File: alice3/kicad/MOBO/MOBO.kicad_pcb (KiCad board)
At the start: 2 copper layers, 97.8 x 114.3 mm, 40 parts, among them CON1 SD_Card, P1 CONN_01X05, SW1 RESET, SW2 SOFT RESET, U1 LM2937-3.3, U2 VGA_daughter_board, U3 Propeller_P8X32A-D40, U4 24LC256, U5 Propeller_Plug, U6 MiniM4-D40, U7 DFROBOT_FTDI_BASIC, U8 Z80CPU, U9 KM681000BLP-7, Y1 5 MHz

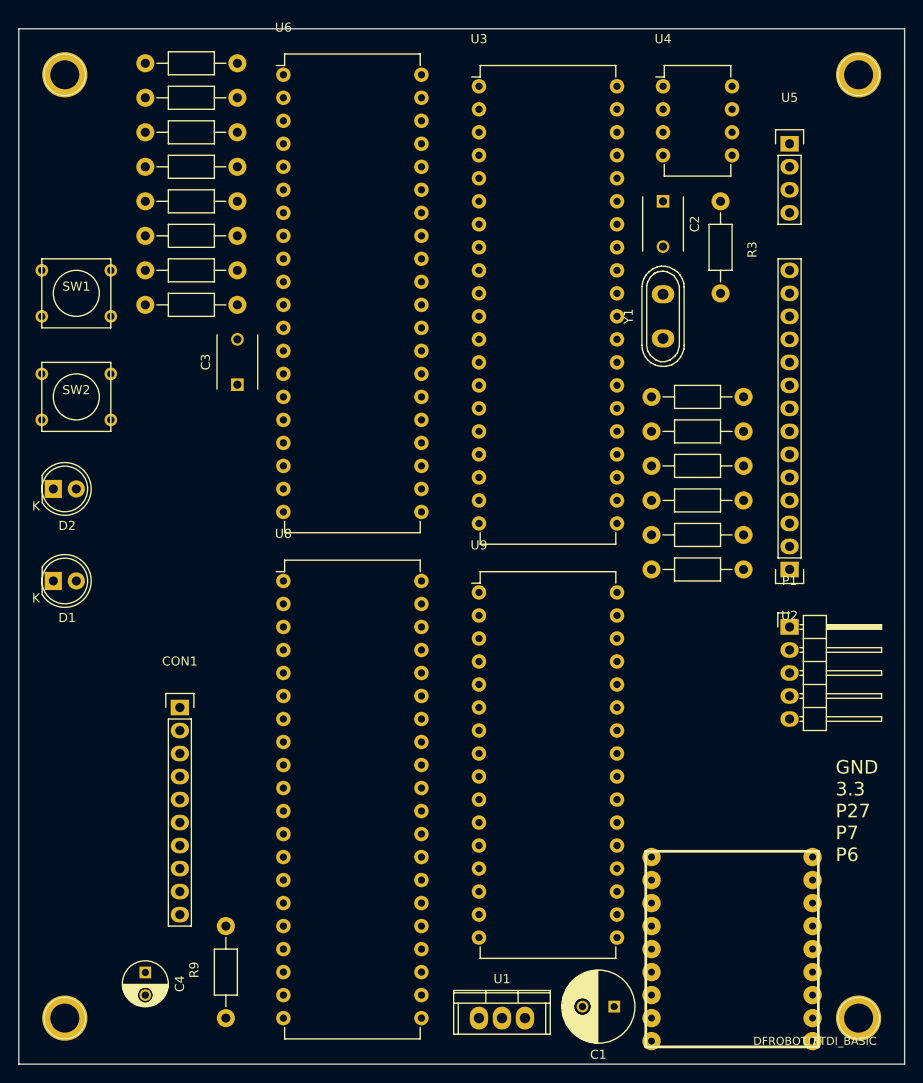
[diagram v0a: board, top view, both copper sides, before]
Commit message: Before removing DFROBOT.
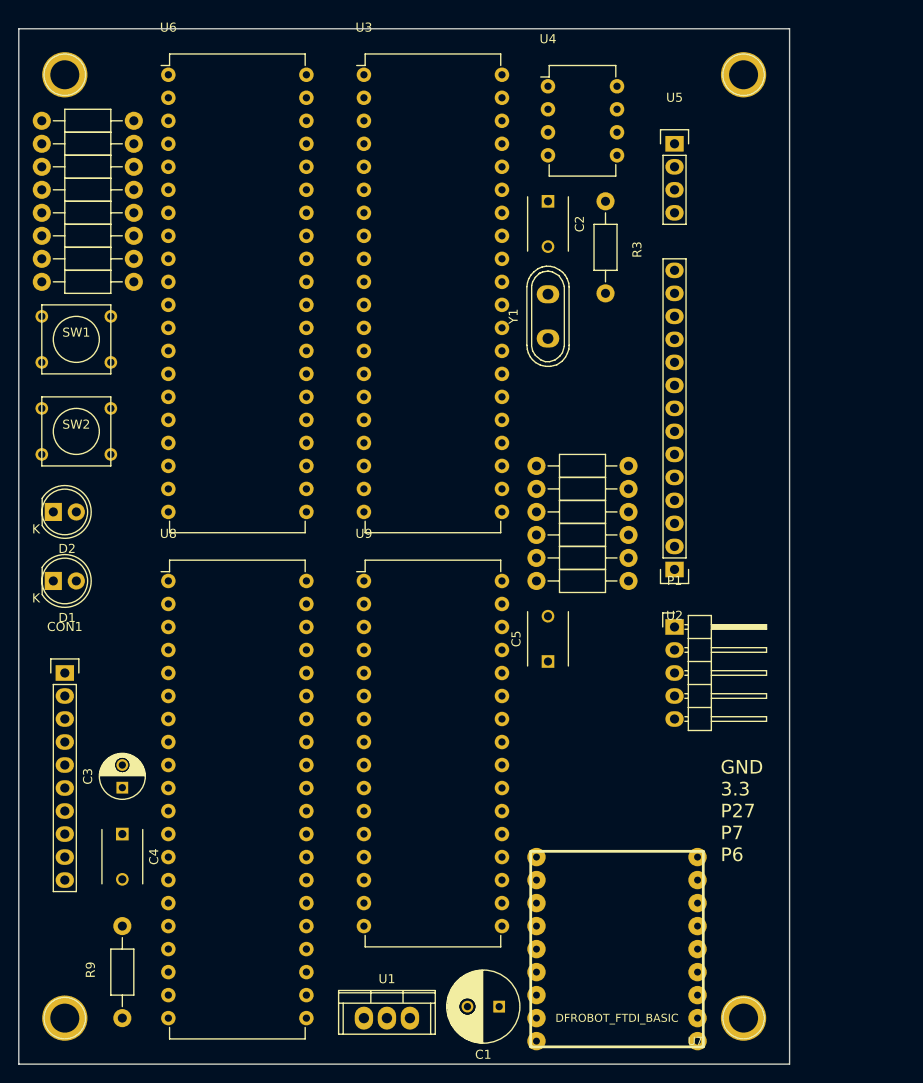
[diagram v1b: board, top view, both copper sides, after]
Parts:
- added C5: 0.1 µF, Capacitors_ThroughHole:C_Disc_D6_P5, F.Cu at (104.1, 102.9)
- C3: value 0.1µ -> 22µF; footprint Capacitors_ThroughHole:C_Disc_D6_P5 -> Capacitors_ThroughHole:C_Radial_D5_L11_P2.5
- C4: value 22µF -> 0.1 µF; footprint Capacitors_ThroughHole:C_Radial_D5_L11_P2.5 -> Capacitors_ThroughHole:C_Disc_D6_P5
- moved C3 46.3 mm to (57.1, 116.8)
- moved C4 15.5 mm to (57.1, 121.9)
- moved R16 14.8 mm to (108.0, 81.3)
- moved R15 14.2 mm to (108.0, 83.8)
- moved R13 13.7 mm to (108.0, 86.4)
- moved CON1 13.3 mm to (50.8, 104.1)
- moved R14 13.3 mm to (108.0, 88.9)
- moved R10 13.1 mm to (53.3, 43.2)
- moved R12 13.0 mm to (108.0, 91.4)
- moved R11 12.8 mm to (108.0, 94.0)
- moved U3 12.8 mm to (83.8, 38.1)
- moved U9 12.8 mm to (83.8, 94.0)
- moved U6 12.7 mm to (62.2, 38.1)
- moved U8 12.7 mm to (62.2, 94.0)
- moved C1 12.7 mm to (98.8, 141.0)
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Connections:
- C4 pad 1: +3V3 -> +5V
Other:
- board size 97.8 x 114.3 mm -> 85.1 x 114.3 mm
